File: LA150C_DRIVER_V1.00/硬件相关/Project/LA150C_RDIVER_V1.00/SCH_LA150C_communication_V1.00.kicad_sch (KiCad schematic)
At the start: 4 parts, among them U3 TCAN3413DDFR

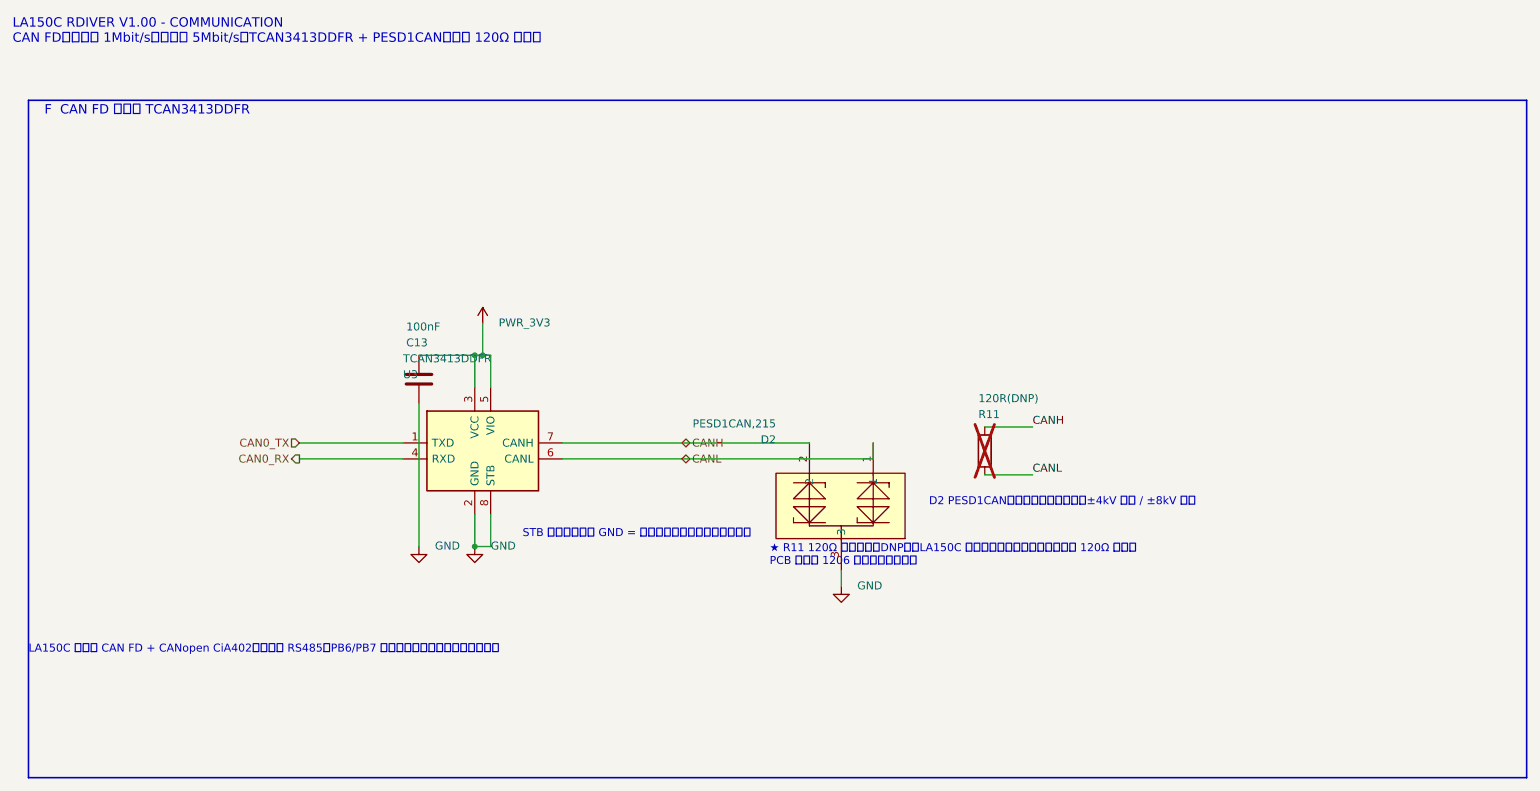
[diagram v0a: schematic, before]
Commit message: chore: save LA150C schematic updates
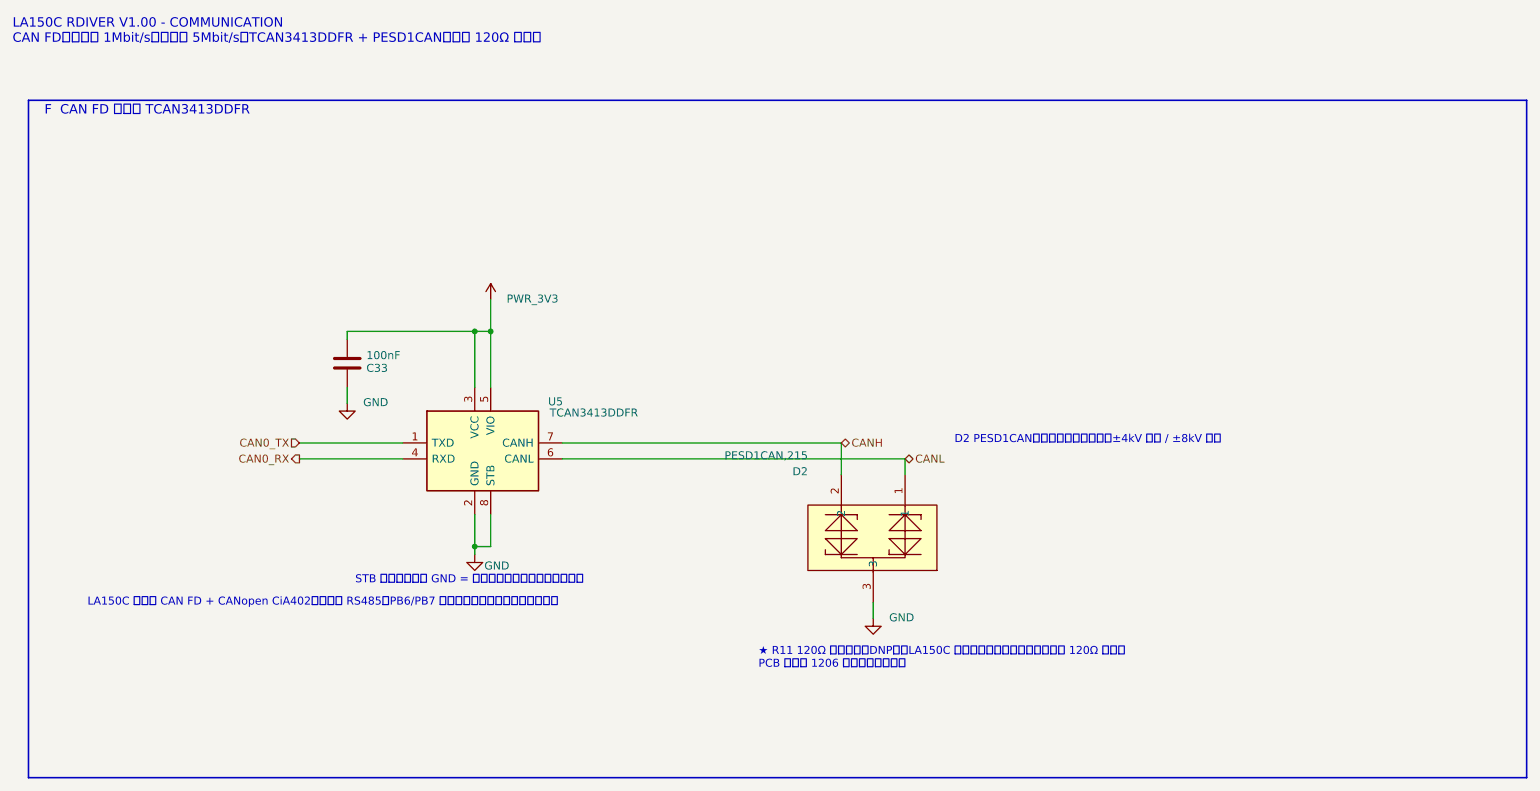
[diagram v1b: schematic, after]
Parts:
- removed R11: 120R(DNP), symbol Device:R
- renumbered C13 to C33, U3 to U5
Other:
- moved on the sheet: C33, D2
